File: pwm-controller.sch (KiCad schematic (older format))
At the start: 39 parts, among them J2 OUT-, J4 POWER, J5 OUT+, J6 DEBUG, J7 I2C, SW1 EC12D1524403, U1 78L05, U3 STM8S003F3Px

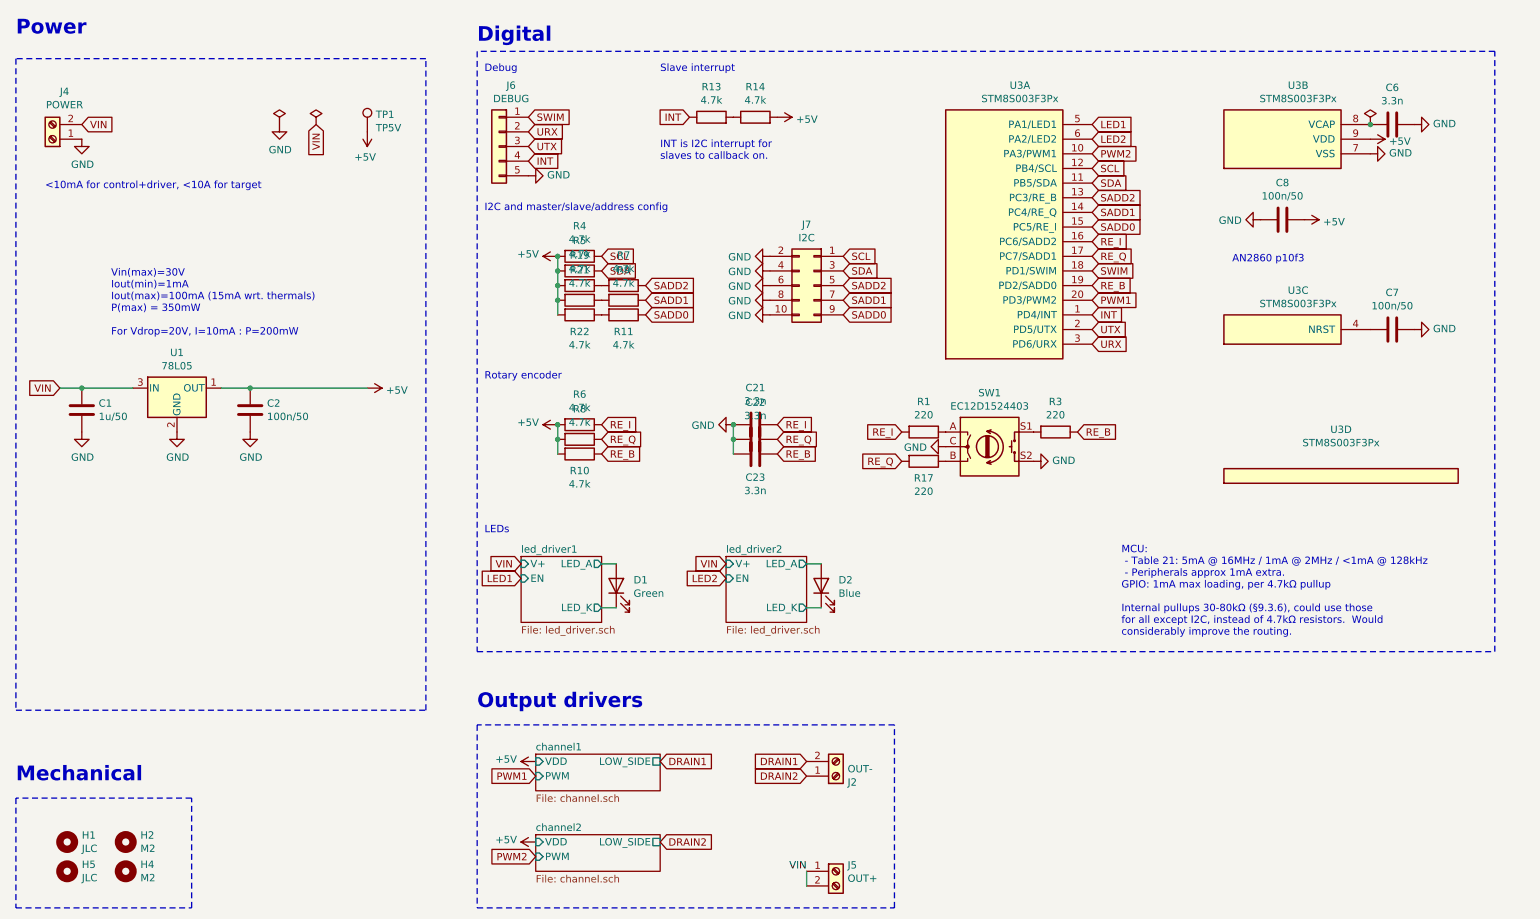
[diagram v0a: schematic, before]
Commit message: ready to order?
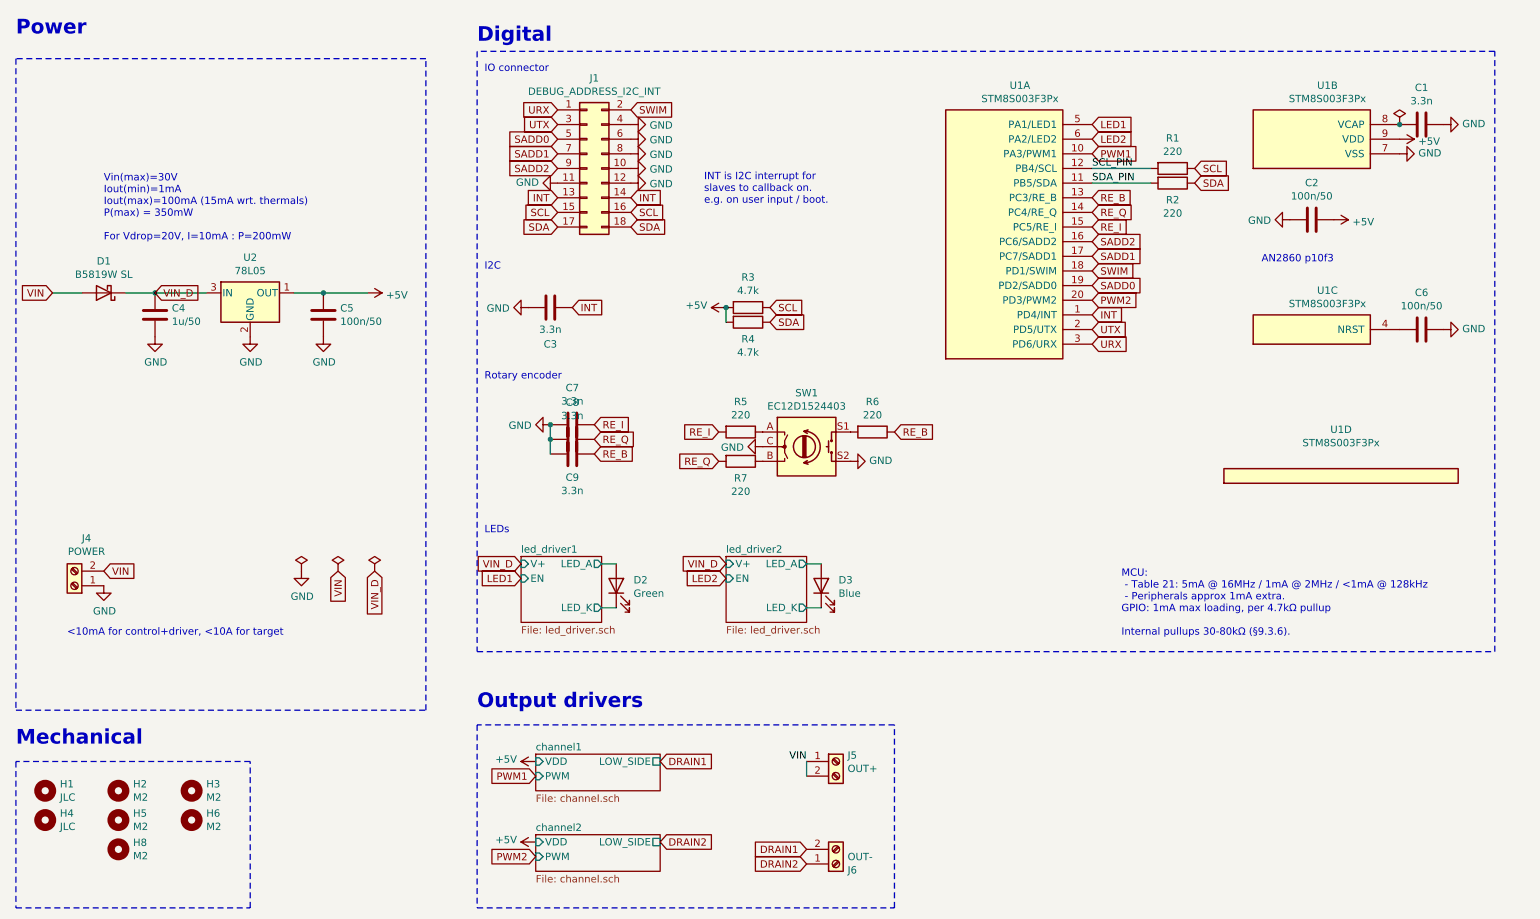
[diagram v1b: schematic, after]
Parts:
- removed J6: DEBUG, Connector_PinHeader_2.54mm:PinHeader_1x05_P2.54mm_Vertical, symbol Connector_Generic:Conn_01x05
- removed J7: I2C, Connector_PinHeader_2.54mm:PinHeader_2x05_P2.54mm_Vertical, symbol Connector_Generic:Conn_02x05_Odd_Even
- removed R10, R11, R13, R14, R19, R21, R22, R6, R7, R8, R9: 4.7k, Resistor_SMD:R_0402_1005Metric, symbol Device:R
- removed TP1: TP5V, TestPoint:TestPoint_Pad_D2.0mm, symbol Connector:TestPoint
- added C3: 3.3n, Capacitor_SMD:C_0402_1005Metric, symbol Device:C
- added D1: B5819W SL, Diode_SMD:D_SOD-123, symbol Device:D_Schottky
- added H3, H6: M2, MountingHole:MountingHole_2mm, symbol Mechanical:MountingHole
- added H8: M2, MountingHole:MountingHole_2.2mm_M2, symbol Mechanical:MountingHole
- added J1: DEBUG_ADDRESS_I2C_INT, Connector_PinHeader_2.54mm:PinHeader_2x09_P2.54mm_Horizontal, symbol Connector_Generic:Conn_02x09_Odd_Even
- added R1, R2: 220, Resistor_SMD:R_0402_1005Metric, symbol Device:R
- renumbered C6 to C1, C8 to C2, C1 to C4, C2 to C5, C7 to C6, C21 to C7, C22 to C8, C23 to C9, D1 to D2, D2 to D3, H5 to H4, H4 to H5, J2 to J6, R4 to R3, R5 to R4, R1 to R5, R3 to R6, R17 to R7, U3 to U1, U1 to U2
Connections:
- net GND: now also C3.1, J1.10 (Pin_10), J1.11 (Pin_11), J1.12 (Pin_12), J1.4 (Pin_4), J1.6 (Pin_6), J1.8 (Pin_8)
- net INT: now also C3.2, J1.13 (Pin_13), J1.14 (Pin_14)
- net PWM1: now also U1.10 (PA3/PWM1); no longer U1.20 (PD3/PWM2)
- net PWM2: now also U1.20 (PD3/PWM2); no longer U1.10 (PA3/PWM1)
- net RE_B: now also U1.13 (PC3/RE_B); no longer U1.19 (PD2/SADD0)
- net RE_I: now also U1.15 (PC5/RE_I); no longer U1.16 (PC6/SADD2)
- net RE_Q: now also U1.14 (PC4/RE_Q); no longer U1.17 (PC7/SADD1)
- net SADD0: now also U1.19 (PD2/SADD0), J1.5 (Pin_5); no longer U1.15 (PC5/RE_I)
- net SADD1: now also U1.17 (PC7/SADD1), J1.7 (Pin_7); no longer U1.14 (PC4/RE_Q)
- net SADD2: now also U1.16 (PC6/SADD2), J1.9 (Pin_9); no longer U1.13 (PC3/RE_B)
- net SCL: now also J1.15 (Pin_15), J1.16 (Pin_16), R1.1; no longer U1.12 (PB4/SCL)
- net SDA: now also J1.17 (Pin_17), J1.18 (Pin_18), R2.1; no longer U1.11 (PB5/SDA)
- net SWIM: now also J1.2 (Pin_2)
- net URX: now also J1.1 (Pin_1)
- net UTX: now also J1.3 (Pin_3)
- net VIN: now also D1.2 (A); no longer C4.1, U2.3 (IN)
- new net SCL_PIN: R1.2, U1.12 (PB4/SCL)
- new net SDA_PIN: R2.2, U1.11 (PB5/SDA)
- new net VIN_D: C4.1, D1.1 (K), U2.3 (IN)
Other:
- note added: "I2C"
- note added: "INT is I2C interrupt for\nslaves to callback on.\ne.g. on user input / boot."
- note added: "IO connector"
- note added: "MCU:\n - Table 21: 5mA @ 16MHz / 1mA @ 2MHz / <1mA @ 128kHz\n - Peripherals approx 1mA extra.\nGPIO: 1mA max loading, per 4.7kΩ pullup\n\nInternal pullups 30-80kΩ (§9.3.6)."
- note removed: "Debug"
- note removed: "I2C and master/slave/address config"
- note removed: "INT is I2C interrupt for\nslaves to callback on."
- note removed: "MCU:\n - Table 21: 5mA @ 16MHz / 1mA @ 2MHz / <1mA @ 128kHz\n - Peripherals approx 1mA extra.\nGPIO: 1mA max loading, per 4.7kΩ pullup\n\nInternal pullups 30-80kΩ (§9.3.6), could use those\nfor all except I2C, instead of 4.7kΩ resistors. Would\nconsiderably improve the routing."
- note removed: "Slave interrupt"
- moved on the sheet: C1, C2, C4, C5, C6, C7, C8, C9, H1, H2, H4, H5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
